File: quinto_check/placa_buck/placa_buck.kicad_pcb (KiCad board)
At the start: 2 copper layers, 126 x 66.5 mm, 52 parts, among them J1 Screw_Terminal_01x02, J2 Screw_Terminal_01x02, J3 Screw_Terminal_01x02, Q1 IRLZ44N, Q2 IRLZ44N, U1 IR2104, U2 TL072, U3 LM393, U4 L7809, U6 LM393, U7 TL072, U8 TL431LP

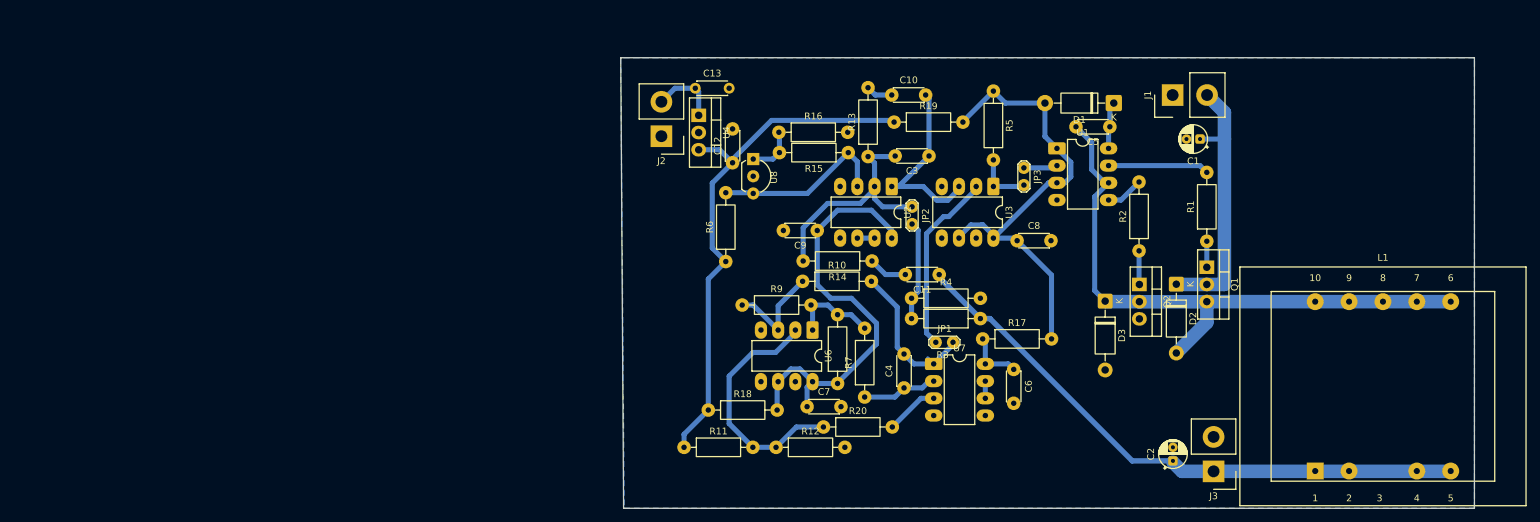
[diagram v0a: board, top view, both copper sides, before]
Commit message: Entrega de quinto check
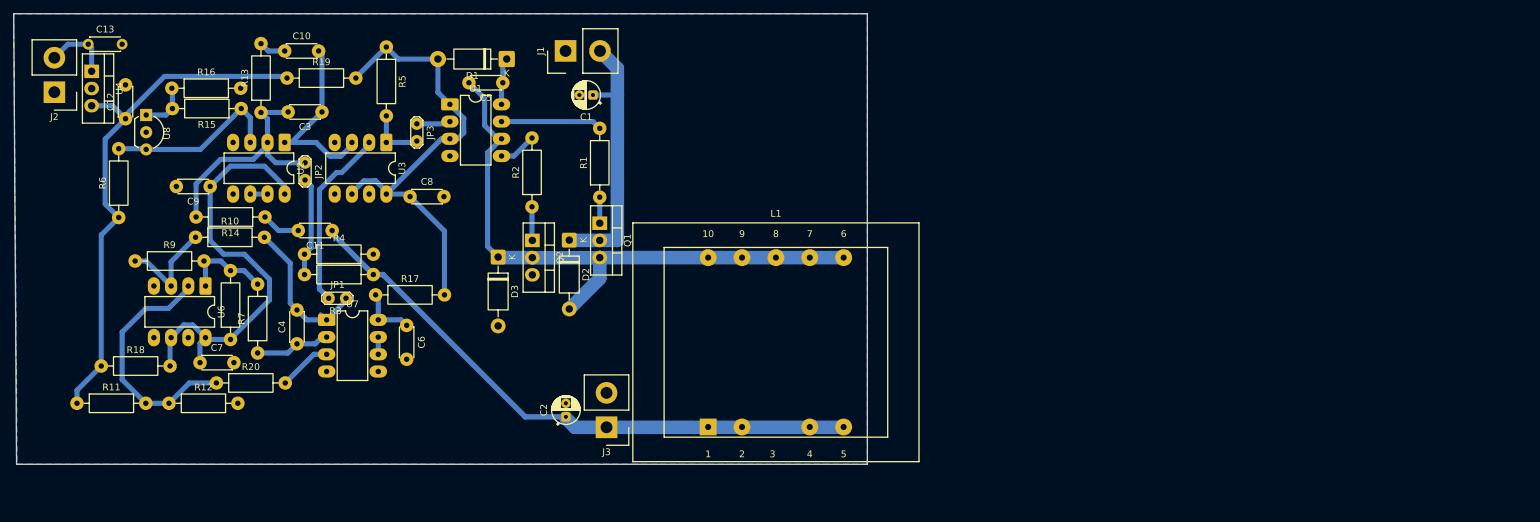
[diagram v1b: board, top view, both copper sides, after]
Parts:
- moved D1 89.8 mm to (113.7, 27.7)
- moved J1 89.8 mm to (122.4, 26.5)
- moved Q2 89.8 mm to (117.4, 54.5)
- moved R14 89.8 mm to (78.0, 51.0)
- moved R15 89.8 mm to (74.5, 35.0)
- moved R3 89.8 mm to (94.0, 59.5)
- moved U8 89.8 mm to (60.4, 36.0)
- moved C1 89.8 mm to (126.4, 33.0)
- moved C10 89.8 mm to (80.9, 26.5)
- moved C11 89.8 mm to (87.9, 53.0)
- moved C12 89.8 mm to (57.4, 36.5)
- moved C13 89.8 mm to (51.9, 25.5)
- moved C2 89.8 mm to (122.4, 80.5)
- moved C3 89.8 mm to (86.4, 35.5)
- moved C4 89.8 mm to (82.7, 69.7)
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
